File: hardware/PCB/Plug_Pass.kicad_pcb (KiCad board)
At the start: 2 copper layers, 47.8 x 73.2 mm, 80 parts, among them IC1 DS3231M, IC2 PN532, IC4 FT232RL, IC5 ATMEGA328P-AUR, J1 USB_B_Micro, J2 505568-0271, J3 Conn_01x08, J4 Conn_01x02, Q1 2N3904, SW1 RESET, Y1 27.12MHz, Y2 ECS-51-20-4

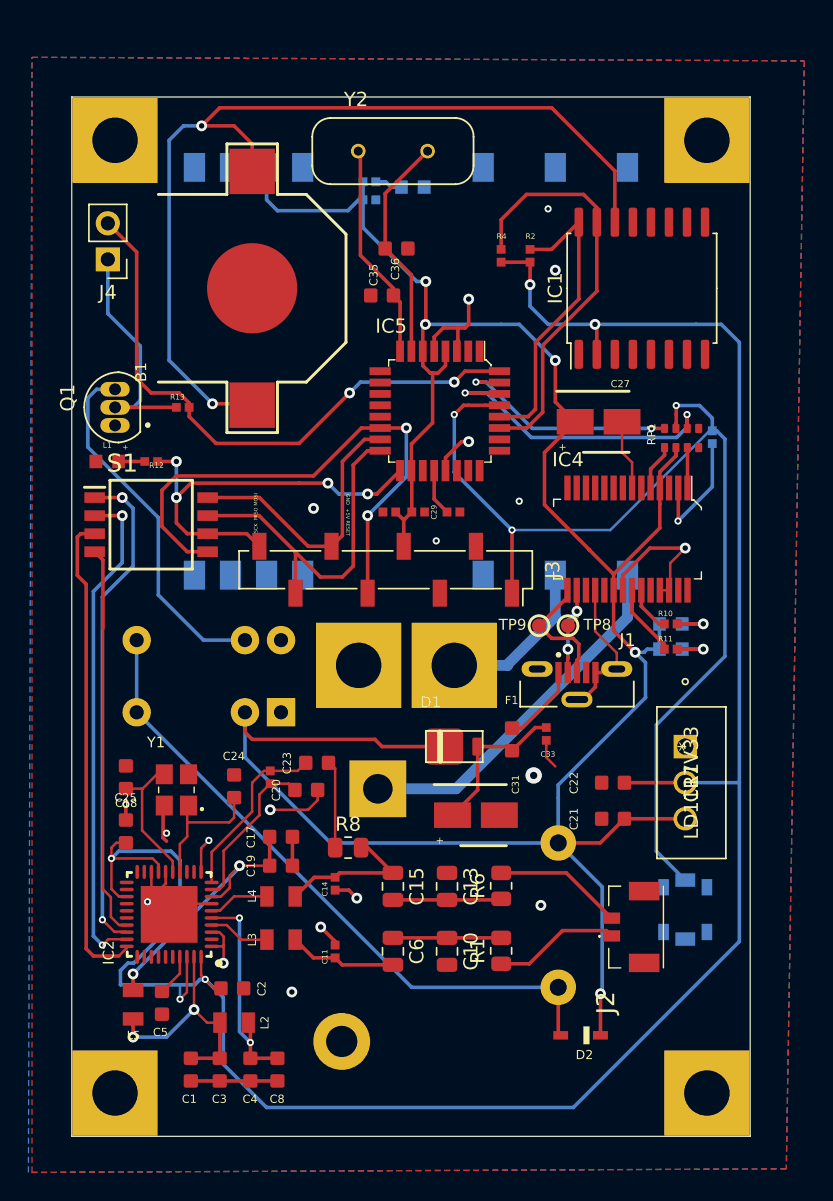
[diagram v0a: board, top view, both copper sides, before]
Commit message: Update 4
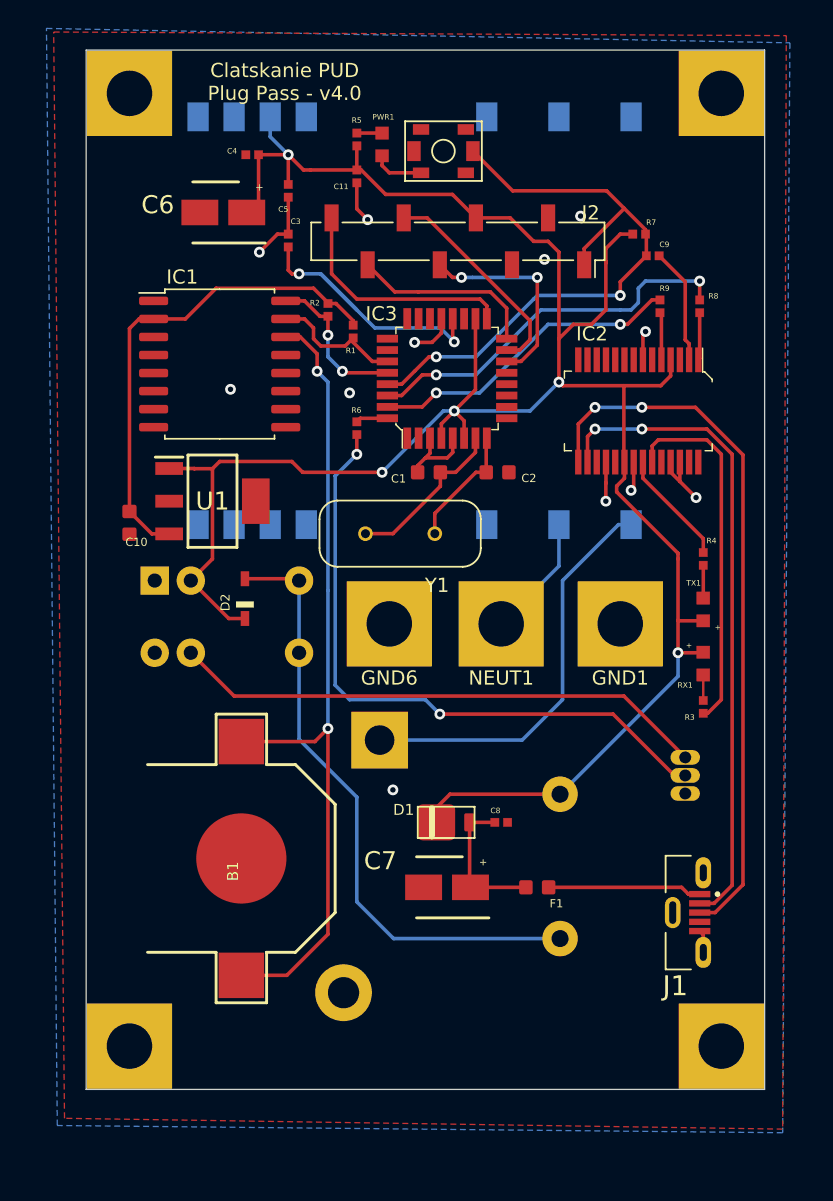
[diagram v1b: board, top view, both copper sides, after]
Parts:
- removed C13: 62pF, Capacitor_SMD:C_0805_2012Metric
- removed C14: 220pF, Plug_Pass:0402-1005X55N
- removed C15: 14pF, Capacitor_SMD:C_0805_2012Metric
- removed C17, C18, C20: 0.1µF, Plug_Pass:0603-1608X90N
- removed C19, C21, C22: 10µF, Plug_Pass:0603-1608X90N
- removed C23: 1000pF, Plug_Pass:0603-1608X90N
- removed C24, C25: 33pF, Plug_Pass:0603-1608X90N
- removed C26, C28: 1µF, Plug_Pass:0402-1005X55N
- removed C27, C31: 4,7uF_16V, Plug_Pass:CAPAE430X550N
- removed C29, C30, C33: 100nF, Plug_Pass:0402-1005X55N
- removed C32: 1uF, Plug_Pass:0402-1005X55N
- removed C35, C36: 22pF, Plug_Pass:0603-1608X90N
- removed CR1: LD1117V33, footprints:LD1117V33
- removed IC4: FT232RL, digikey-footprints:SSOP-28_W5.30mm
- removed IC5: ATMEGA328P-AUR, digikey-footprints:TQFP-32_7x7mm
- removed J3: Conn_01x08, Connector_PinSocket_2.54mm:PinSocket_1x08_P2.54mm_Vertical_SMD_Pin1Right
- removed J4: Conn_01x02, Connector_PinHeader_2.54mm:PinHeader_1x02_P2.54mm_Vertical
- removed L1: Yellow, Plug_Pass:LEDC1608X80N-AK
- removed L2, L5: FERRITE, Plug_Pass:0805-R2013X50N
- removed L3, L4: 560nH, Plug_Pass:0805-R2013X50N
- removed R10, R11, R12: 330, Plug_Pass:0402-1005X55N
- removed R13: 4.7k, Plug_Pass:0402-1005X55N
- removed RP1: 1k, Plug_Pass:CAY16
- removed S1: 218-4LPST, Plug_Pass:SOIC127P844X265-8N
- removed TP8: D11, Plug_Pass:TESTPOINT_ROUND_1MM
- removed TP9: D+1, Plug_Pass:TESTPOINT_ROUND_1MM
- removed Y2: ECS-51-20-4, ECS-51-20-4:XTAL_ECS-51-20-4
- added C7: 4.7uF, Plug_Pass:CAPAE430X550N, F.Cu at (155.4, 109.0)
- added C9: 100nF, Plug_Pass:0402-1005X55N, F.Cu at (169.9, 64.5)
- added GND6: GND, Plug_Pass:Ground_Pad, F.Cu at (151.4, 90.4)
- added IC3: ATMEGA328P-AUR, Plug_Pass:TQFP-32_7x7mm, F.Cu at (155.4, 73.2)
- added R3: 330, Plug_Pass:0402-1005X55N, F.Cu at (173.5, 96.3)
- added R5: 330, Plug_Pass:0402-1005X55N, F.Cu at (149.1, 56.3)
- added U1: TC1108-3.3VDBTR, SamacSys_Parts:SOT230P700X180-4N, F.Cu at (138.9, 81.8)
- C1, C2: value 0.1µF -> 22pF
- C10: value 62pF -> 1µF; footprint Capacitor_SMD:C_0805_2012Metric -> Plug_Pass:0603-1608X90N
- C11: value 220pF -> 1uF
- C3, C8: value 0.1µF -> 100nF; footprint Plug_Pass:0603-1608X90N -> Plug_Pass:0402-1005X55N
- C4, C5: value 10µF -> 1µF; footprint Plug_Pass:0603-1608X90N -> Plug_Pass:0402-1005X55N
- C6: value 14pF -> 4.7uF; footprint Capacitor_SMD:C_0805_2012Metric -> Plug_Pass:CAPAE430X550N
- IC2: value PN532 -> FT232RL; footprint Plug_Pass:HVQFN40-6X6 -> Plug_Pass:SSOP-28_W5.30mm
- J2: value 505568-0271 -> Conn_01x08; footprint Plug_Pass:5055680271 -> Connector_PinSocket_2.54mm:PinSocket_1x08_P2.54mm_Vertical_SMD_Pin1Right
- PWR1, RX1, SW1, TX1: moved to F.Cu
- Q1: moved to B.Cu
- R1: value 2 -> 10k; footprint Resistor_SMD:R_0805_2012Metric -> Plug_Pass:0402-1005X55N
- R4: value 10k -> 330
- R6: value 2 -> 4.7k; footprint Resistor_SMD:R_0805_2012Metric -> Plug_Pass:0402-1005X55N
- R7: value 1.0k -> 1k
- R8: value 1.69k -> 1k; footprint Resistor_SMD:R_0805_2012Metric -> Plug_Pass:0402-1005X55N
- R9: value 330 -> 1k; moved to F.Cu
- Y1: value 27.12MHz -> ECS-51-20-4; footprint Plug_Pass:7M27120MAAJT -> ECS-51-20-4:XTAL_ECS-51-20-4
- moved C4 64.4 mm to (141.7, 57.4), turned to 180 degrees
- moved C3 58.6 mm to (144.3, 63.4)
- moved C5 57.8 mm to (144.3, 59.9)
- moved SW1 56.0 mm to (155.2, 57.1), turned to 0 degrees
- moved C11 54.6 mm to (149.1, 58.9), turned to 270 degrees
- moved C6 53.4 mm to (139.7, 61.5), turned to 180 degrees
- moved J2 49.8 mm to (156.2, 63.5)
- moved IC2 48.4 mm to (168.9, 75.4)
- moved Q1 47.8 mm to (172.2, 101.1)
- moved R7 46.2 mm to (169.0, 63.0), turned to 180 degrees
- moved R8 45.4 mm to (173.2, 68.1), turned to 270 degrees
- moved C1 45.3 mm to (154.2, 79.8), turned to 0 degrees
- moved R1 44.8 mm to (148.8, 69.8)
- moved C2 40.8 mm to (159.0, 79.8)
- moved B1 40.1 mm to (141.0, 106.9)
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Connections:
- C1 pad 1: LDO -> GNDREF
- C1 pad 2: GNDREF -> Net-(C1-Pad2)
- C10 pad 1: Net-(C10-Pad1) -> +3V3
- C11 pad 1: Net-(C11-Pad1) -> +5V
- C2 pad 2: +3V3 -> Net-(C2-Pad2)
- C3 pad 1: GNDREF -> Net-(C3-Pad1)
- C3 pad 2: LDO -> GNDREF
- C4 pad 1: GNDREF -> +5V
- C4 pad 2: /TVDD -> GNDREF
- C5 pad 1: Net-(C5-Pad1) -> +5V
- C6 pad 1: Net-(C10-Pad1) -> +5V
- C6 pad 2: Net-(C11-Pad1) -> GNDREF
- C8 pad 1: GNDREF -> Net-(C7-Pad1)
- C8 pad 2: /TVDD -> GNDREF
- D1 pad P$2: Net-(C31-Pad1) -> Net-(C7-Pad1)
- F1 pad 2: Net-(C31-Pad1) -> Net-(C7-Pad1)
- IC1 pad 1: /32K -> (no net)
- IC1 pad 3: /SQW -> (no net)
- IC1 pad 4: Net-(IC1-Pad4) -> (no net)
- IC2 pad 1: GNDREF -> RX
- IC2 pad 10: /RX1 -> (no net)
- IC2 pad 11: GNDREF -> (no net)
- IC2 pad 12: Net-(IC2-Pad12) -> (no net)
- IC2 pad 13: Net-(IC2-Pad13) -> (no net)
- IC2 pad 14: Net-(C24-Pad1) -> (no net)
- IC2 pad 15: Net-(C25-Pad1) -> /D+
- IC2 pad 16: GNDREF -> /D-
- IC2 pad 17: +3V3 -> (no net)
- IC2 pad 19: Net-(IC2-Pad19) -> (no net)
- IC2 pad 20: Net-(IC2-Pad20) -> +5V
- IC2 pad 21: Net-(IC2-Pad21) -> GNDREF
- IC2 pad 22: Net-(IC2-Pad22) -> /TX_GREEN
- IC2 pad 23: +3V3 -> /RX_RED
- IC2 pad 24: Net-(IC2-Pad24) -> (no net)
- IC2 pad 25: Net-(IC2-Pad25) -> GNDREF
- IC2 pad 26: Net-(IC2-Pad26) -> GNDREF
- IC2 pad 27: SS-1 -> (no net)
- IC2 pad 28: MOSI-1 -> (no net)
- IC2 pad 3: GNDREF -> (no net)
- IC2 pad 4: /TX1 -> +5V
- IC2 pad 5: /TVDD -> TX
- IC2 pad 6: /TX2 -> (no net)
- IC2 pad 8: /AVDD -> (no net)
- IC2 pad 9: /VMID -> (no net)
- J1 pad 4: Net-(J1-Pad4) -> (no net)
- J2 pad 1: Net-(J2-Pad1) -> RESET
- J2 pad 2: Net-(J2-Pad2) -> GNDREF
- J2 pad 4: GNDREF -> +5V
- Q1 pad 2: Net-(J4-Pad1) -> Net-(Q1-Pad2)
- R1 pad 1: Net-(J2-Pad1) -> SDA
- R1 pad 2: Net-(C10-Pad1) -> +3V3
- R4 pad 1: SDA -> /TX_GREEN
- R4 pad 2: +3V3 -> Net-(R4-Pad2)
- R6 pad 1: Net-(C13-Pad2) -> Net-(Q1-Pad2)
- R6 pad 2: Net-(J2-Pad2) -> RLY
- R7 pad 1: /RX1 -> RESET
- R7 pad 2: /VMID -> +5V
- R8 pad 2: Net-(C14-Pad2) -> RX
- R9 pad 1: +5V -> Net-(IC3-Pad31)
- R9 pad 2: Net-(PWR1-PadA) -> TX
- RLY1 pad 3: Net-(RLY1-Pad3) -> (no net)
- RLY2 pad 1: Net-(RLY2-Pad1) -> (no net)
- TX1 pad C: Net-(R11-Pad2) -> Net-(R4-Pad2)
- Y1 pad 1: Net-(C24-Pad1) -> Net-(C2-Pad2)
- Y1 pad 2: GNDREF -> Net-(C1-Pad2)
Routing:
- net +3V3: track 161.2 -> 34.5 mm, vias 5 -> 0
- net Net-(Q1-Pad2): track 0.00 -> 46.1 mm, vias 0 -> 2
- net GNDREF: track 76.6 -> 34.4 mm, vias 19 -> 12
- net /D+: track 8.72 -> 50.2 mm, vias 0 -> 2
- net RLY: track 41.9 -> 2.25 mm, vias 2 -> 0
- net /D-: track 7.35 -> 46.1 mm
- net MISO-1: track 35.2 -> 0.00 mm, vias 2 -> 0
- net MOSI-1: track 34.9 -> 0.00 mm, vias 2 -> 0
- net SCK-1: track 34.0 -> 0.00 mm
- net RESET: track 75.1 -> 44.0 mm, vias 3 -> 2
- net SS-1: track 27.5 -> 0.00 mm
- net SS: track 38.3 -> 14.6 mm
- net Net-(IC3-Pad31): track 0.00 -> 22.3 mm, vias 0 -> 2
- net /RX_RED: track 3.27 -> 25.5 mm
- net Net-(IC5-Pad30): track 21.7 -> 0.00 mm, vias 2 -> 0
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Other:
- board text added: "Clatskanie PUD Plug Pass - v4.0"
- board text removed: "+5V"
- board text removed: "Clatskanie PUD Plug Pass - v3.2"
- board text removed: "GND"
- board text removed: "MISO"
- board text removed: "MOSI"
- board text removed: "RESET"
- board text removed: "SCK"
